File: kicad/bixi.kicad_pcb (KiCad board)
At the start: 2 copper layers, 100 x 100 mm, 34 parts, among them CON1 BARREL_JACK, J1 RJ45, J2 RJ45, J3 RJ45, J4 RJ45, J5 RJ45, J6 RJ45, J7 RJ45, J8 RJ45, U1 Teensy3.6, U2 SP3485CN, U3 SP3485CN, U4 SP3485CN, U5 SP3485CN, U6 SP3485CN, U7 SP3485CN, U8 SP3485CN, U9 SP3485CN

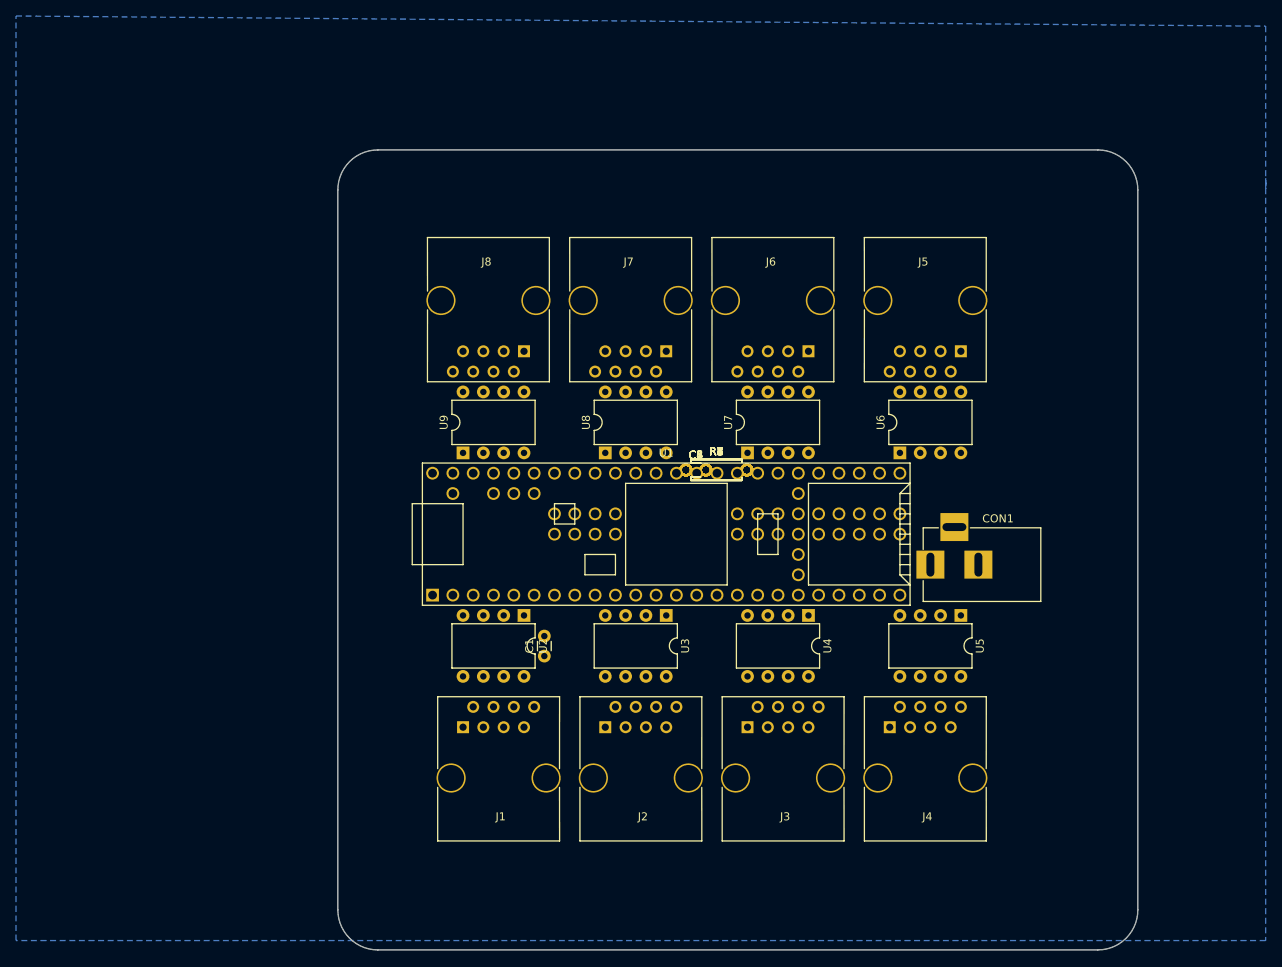
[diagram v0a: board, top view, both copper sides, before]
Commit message: kicad schematic and layout
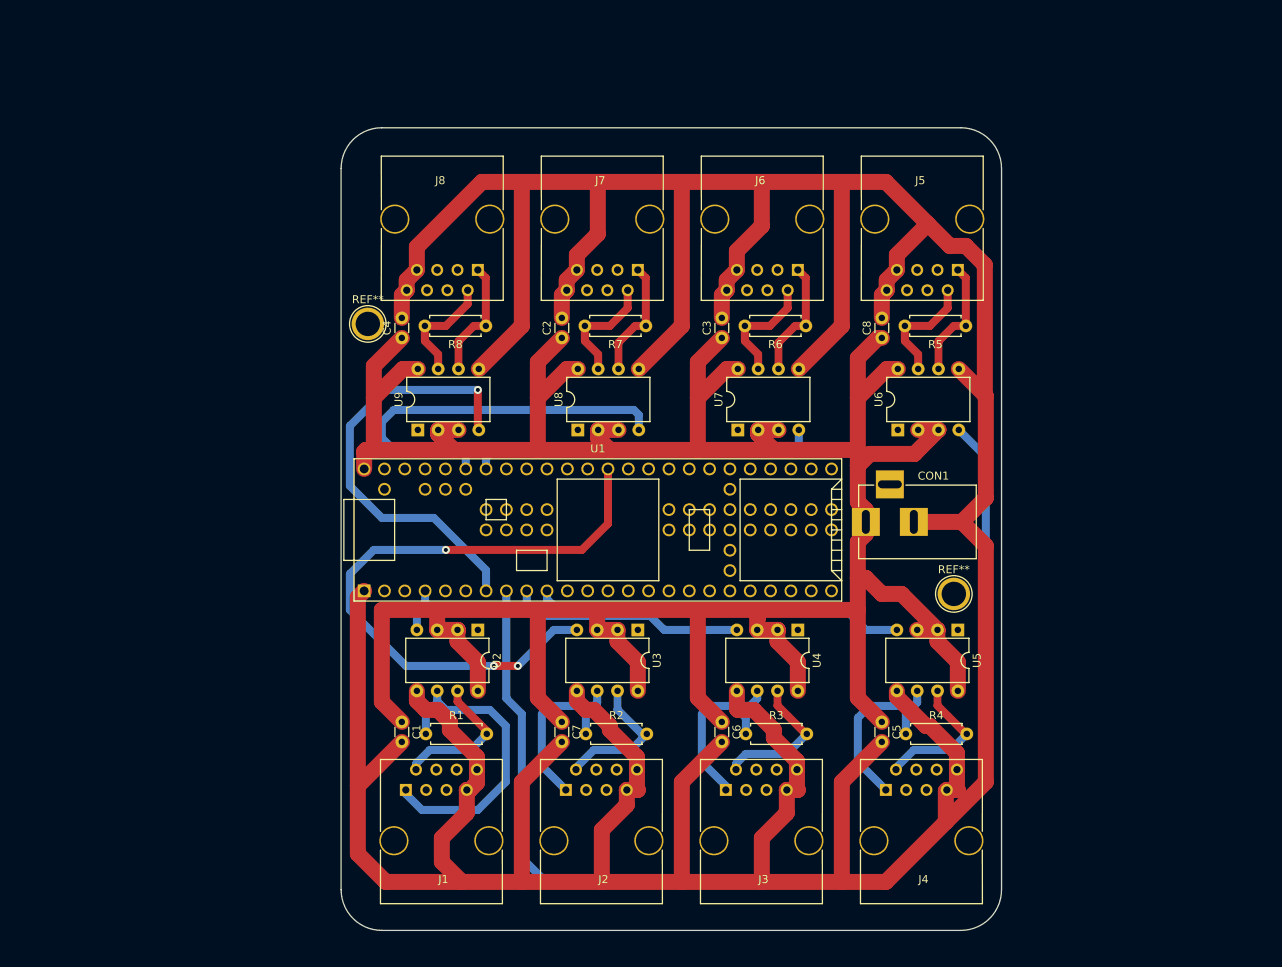
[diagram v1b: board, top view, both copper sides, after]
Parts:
- added REF**: 1pin, Connectors:1pin, F.Cu at (182.0, 120.5)
- added REF**: 1pin, Connectors:1pin, F.Cu at (108.8, 86.8)
- moved R1 46.3 mm to (116.0, 138.0)
- moved R4 43.0 mm to (176.0, 138.0)
- moved C5 39.9 mm to (173.0, 136.5), turned to 270 degrees
- moved R5 39.4 mm to (183.5, 87.0), turned to 180 degrees
- moved C4 39.1 mm to (113.0, 88.5), turned to 90 degrees
- moved R2 35.3 mm to (136.0, 138.0)
- moved C7 35.1 mm to (133.0, 136.5), turned to 270 degrees
- moved R3 33.8 mm to (156.0, 138.0)
- moved C6 31.8 mm to (153.0, 136.5), turned to 270 degrees
- moved R8 30.8 mm to (123.5, 87.0), turned to 180 degrees
- moved C8 29.5 mm to (173.0, 88.5), turned to 90 degrees
- moved R6 23.4 mm to (163.5, 87.0), turned to 180 degrees
- moved C2 22.6 mm to (133.0, 88.5), turned to 90 degrees
- moved C1 19.6 mm to (113.0, 136.5), turned to 270 degrees
- moved R7 18.7 mm to (143.5, 87.0), turned to 180 degrees
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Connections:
- U1 pad 53: Net-(U1-Pad53) -> VCC
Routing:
- net GND: track 0.00 -> 593.2 mm
- net VCC: track 0.00 -> 396.1 mm
- net /WS_5: track 0.00 -> 144.0 mm
- net /WS_2: track 0.00 -> 79.4 mm, vias 0 -> 3
- net /WS_8: track 0.00 -> 54.4 mm, vias 0 -> 1
- net /WS_7: track 0.00 -> 50.1 mm
- net /WS_4: track 0.00 -> 46.4 mm
- net /WS_6: track 0.00 -> 43.0 mm
- net Net-(J1-Pad1): track 0.00 -> 38.1 mm
- net /WS_3: track 0.00 -> 29.3 mm
- net Net-(J4-Pad1): track 0.00 -> 24.0 mm
- net Net-(J2-Pad1): track 0.00 -> 23.6 mm
- net Net-(J3-Pad1): track 0.00 -> 23.5 mm
- net Net-(J3-Pad2): track 0.00 -> 18.1 mm
- net Net-(J2-Pad2): track 0.00 -> 18.1 mm
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- removed copper zone on B.Cu, net GND
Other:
- board size 100 x 100 mm -> 82.6 x 100.3 mm
- net class Default: trace_width 0.25 -> 1; via_dia 0.6 -> 1; via_drill 0.4 -> 0.5
